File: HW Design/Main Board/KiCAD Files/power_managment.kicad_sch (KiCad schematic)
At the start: 3 parts, among them U1 LM3940IMP-3.3/NOPB

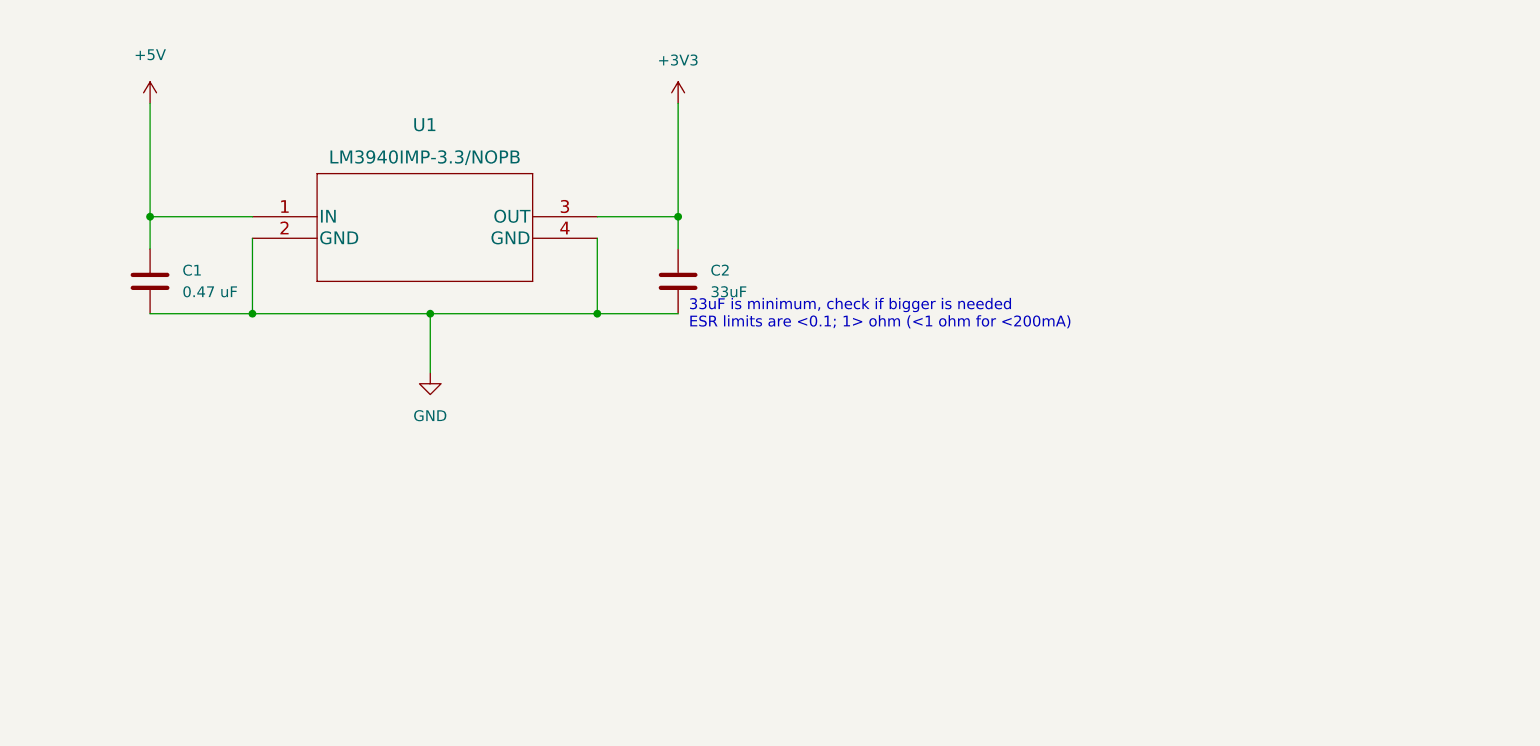
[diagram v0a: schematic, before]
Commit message: hw desgign updates
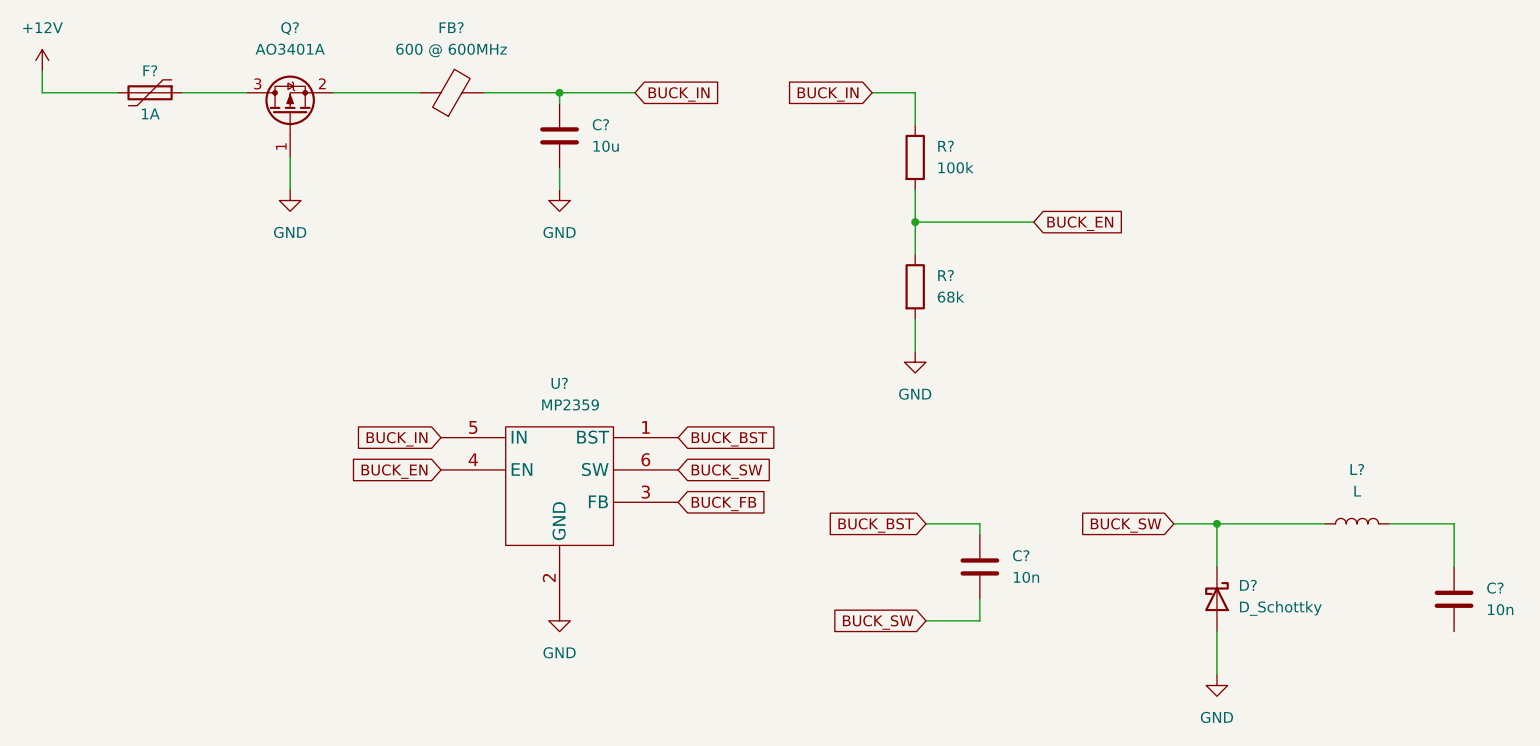
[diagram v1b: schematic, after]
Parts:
- removed C1: 0.47 uF, symbol Device:C
- removed C2: 33uF, symbol Device:C
- removed U1: LM3940IMP-3.3/NOPB, Package_TO_SOT_SMD:SOT-223, symbol LM3940:LM3940IMP-3.3/NOPB
- added C? (x2): 10n, symbol Device:C
- added C?: 10u, symbol Device:C
- added D?: D_Schottky, symbol Device:D_Schottky
- added F?: 1A, symbol Device:Polyfuse
- added FB?: 600 @ 600MHz, symbol Device:FerriteBead
- added L?: L, symbol Device:L
- added Q?: AO3401A, Package_TO_SOT_SMD:SOT-23, symbol Transistor_FET:AO3401A
- added R?: 68k, symbol Device:R
- added R?: 100k, symbol Device:R
- added U?: MP2359, symbol New_Library:MP2359
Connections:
- net GND: now also C?.2, D?.2 (A), Q?.1 (G), R?.2, U?.2 (GND)
- new net: C?.1, L?.2
- new net: FB?.1, Q?.2 (S)
- new net: F?.1, Q?.3 (D)
- new net +12V: F?.2
- new net BUCK_BST: C?.1, U?.1 (BST)
- new net BUCK_EN: R?.1, R?.2, U?.4 (EN)
- new net BUCK_FB: U?.3 (FB)
- new net BUCK_IN: C?.1, FB?.2, R?.1, U?.5 (IN)
- new net BUCK_SW: C?.2, D?.1 (K), L?.1, U?.6 (SW)
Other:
- note removed: "33uF is minimum, check if bigger is needed ESR limits are <0.1; 1> ohm (<1 ohm for <200mA)"
